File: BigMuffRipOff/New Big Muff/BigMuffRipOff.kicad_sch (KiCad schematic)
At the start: 9 parts, among them J2 NMJ6HFD2, J3 NMJ6HFD2, J4 2125201004, J6 2125201004, J7 2125201004

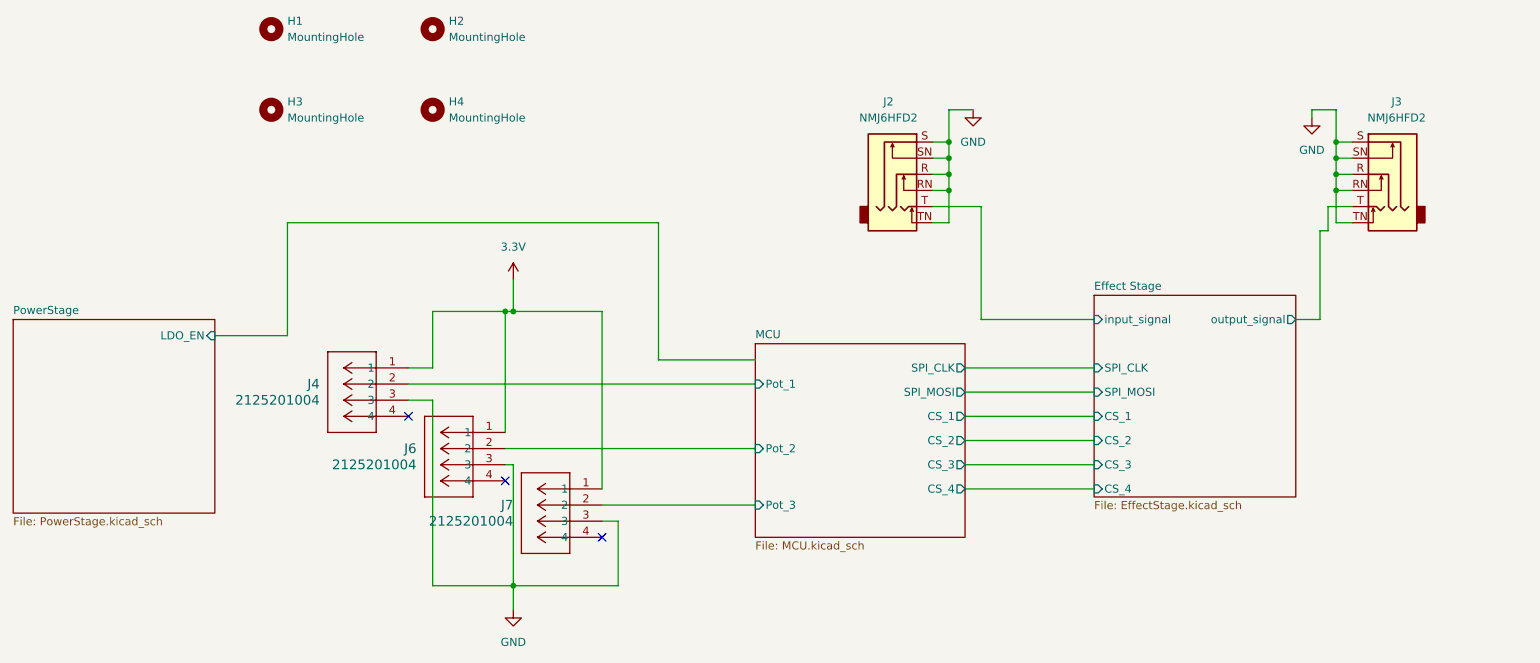
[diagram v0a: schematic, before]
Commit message: new big muff completed
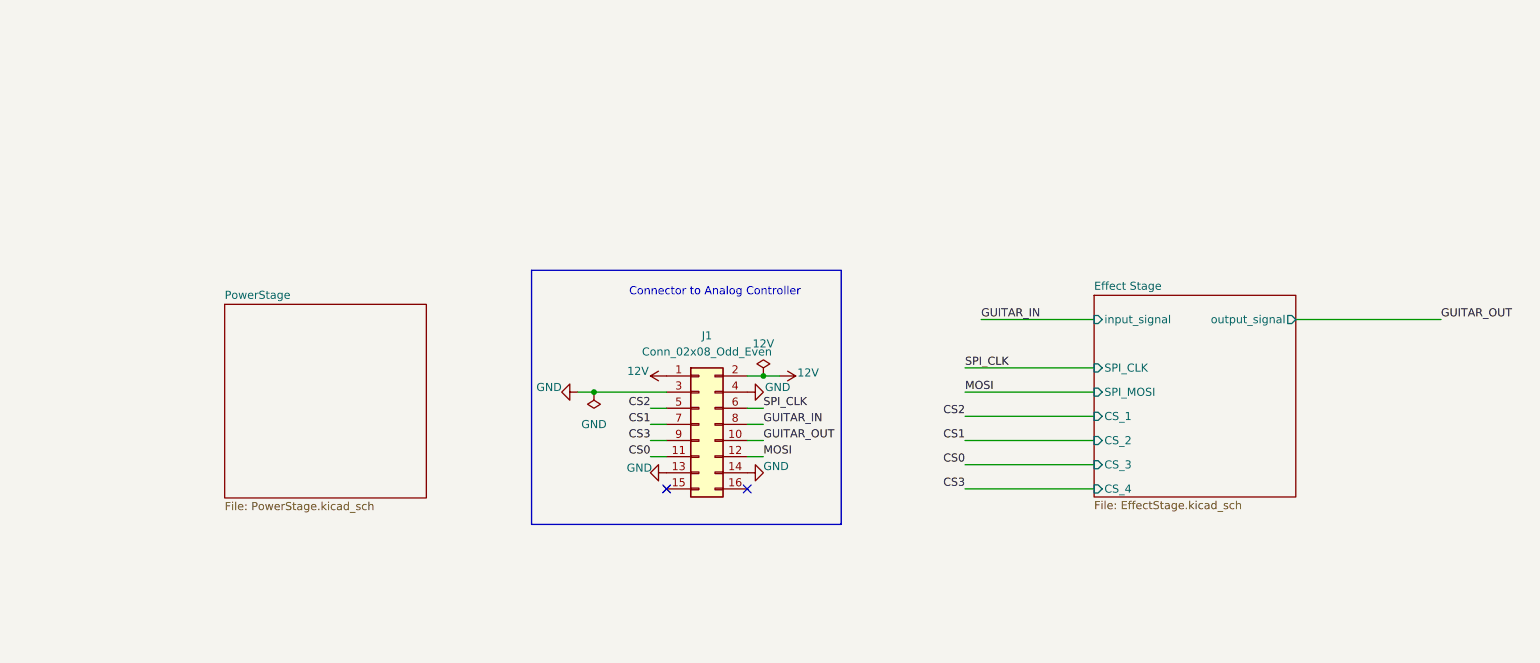
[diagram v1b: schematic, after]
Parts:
- removed H1, H2, H3, H4: MountingHole, MountingHole:MountingHole_2.2mm_M2, symbol Mechanical:MountingHole
- removed J2, J3: NMJ6HFD2, Connector_Audio:Jack_6.35mm_Neutrik_NMJ6HFD2_Horizontal, symbol Connector_Audio:NMJ6HFD2
- removed J4, J6, J7: 2125201004, 284867-E-footprint:CONN_2125200001-SD_04_MOL, symbol Molex 4pin header vert:2125201004
- added J1: Conn_02x08_Odd_Even, Connector_PinHeader_2.54mm:PinHeader_2x08_P2.54mm_Horizontal, symbol Connector_Generic:Conn_02x08_Odd_Even
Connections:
- net GND: now also J1.13 (Pin_13), J1.14 (Pin_14), J1.3 (Pin_3), J1.4 (Pin_4)
- new net 12V: J1.1 (Pin_1), J1.2 (Pin_2)
- new net CS0: J1.11 (Pin_11)
- new net CS1: J1.7 (Pin_7)
- new net CS2: J1.5 (Pin_5)
- new net CS3: J1.9 (Pin_9)
- new net GUITAR_IN: J1.8 (Pin_8)
- new net GUITAR_OUT: J1.10 (Pin_10)
- new net MOSI: J1.12 (Pin_12)
- new net SPI_CLK: J1.6 (Pin_6)
- no-connect marks 3 -> 2
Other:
- removed sheet MCU
- sheet PowerStage ports: added none; removed LDO_EN
- note added: "Connector to Analog Controller"
